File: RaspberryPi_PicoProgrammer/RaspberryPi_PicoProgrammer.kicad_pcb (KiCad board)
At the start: 2 copper layers, 43.2 x 27.9 mm, 7 parts, among them J1 Conn_02x05_Odd_Even, J2 Conn_01x07_Male, J3 Conn_02x03_Odd_Even, J4 BM03B-SRSS-TBLFSN, U1 Pico

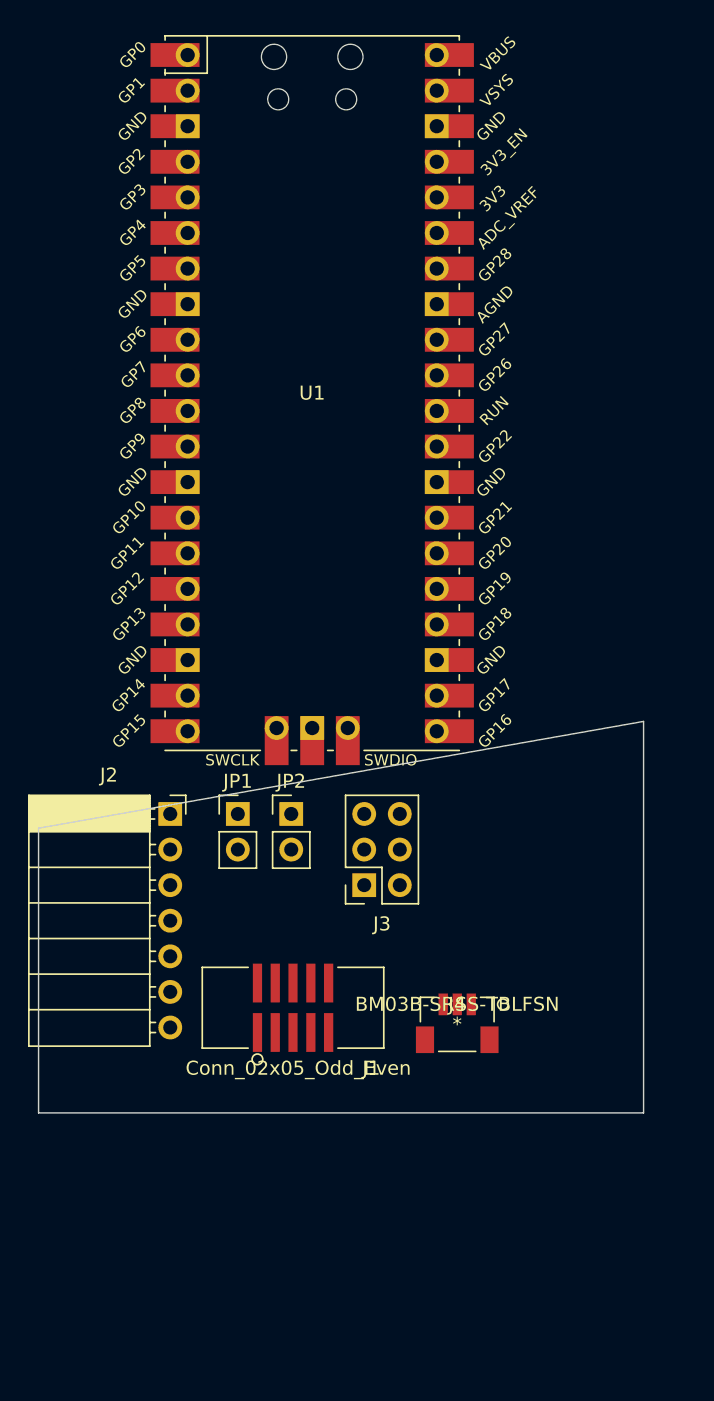
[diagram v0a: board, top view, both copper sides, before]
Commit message: added schematic for raspberry pi
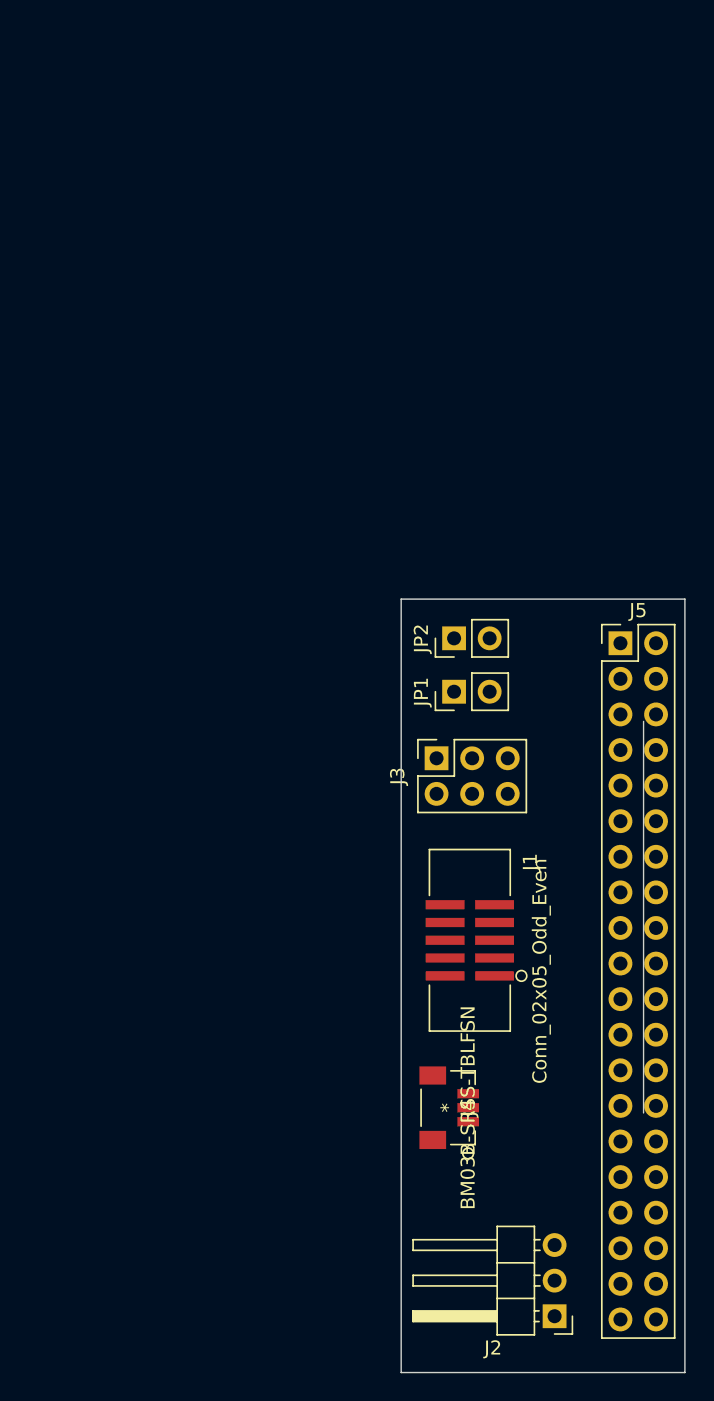
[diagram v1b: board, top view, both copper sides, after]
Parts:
- removed U1: Pico, MCU_RaspberryPi_and_Boards:RPi_Pico_SMD_TH
- added J5: Raspberry_Pi_2_3, Connector_PinHeader_2.54mm:PinHeader_2x20_P2.54mm_Vertical, F.Cu at (150.8, 63.0)
- J2: value Conn_01x07_Male -> Conn_01x03_Male; footprint Connector_PinSocket_2.54mm:PinSocket_1x07_P2.54mm_Horizontal -> Connector_PinHeader_2.54mm:PinHeader_1x03_P2.54mm_Horizontal
- moved J2 45.1 mm to (146.1, 111.0), turned to 180 degrees
- moved JP1 17.7 mm to (138.9, 66.5), turned to 90 degrees
- moved JP2 17.1 mm to (138.9, 62.6), turned to 90 degrees
- moved J1 13.5 mm to (140.0, 84.2), turned to 90 degrees
- moved J3 10.4 mm to (137.6, 71.2), turned to 90 degrees
- moved J4 5.99 mm to (138.4, 96.2), turned to -90 degrees
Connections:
- J2 pad 1: /SCL_0 -> /SWDCLK
- J2 pad 2: /SWDCLK -> Earth
- J2 pad 3: Earth -> /SWO
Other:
- board size 43.2 x 27.9 mm -> 20.2 x 55.2 mm
